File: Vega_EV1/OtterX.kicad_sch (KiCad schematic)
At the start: 62 parts, among them J1 VERA_CONN, J11 KMDGX-6SG, J12 VIA1 Extra Pins, J17 SNES23, J18 SNES0, J19 SNES1, J2 VIA2 Header, J29 AudioPlug3, J3 IEC, J9 I2C, U1 W65C02S, U11 74ACT163, U2 W65C22S, X1 ACH-16.000MHZ-EK

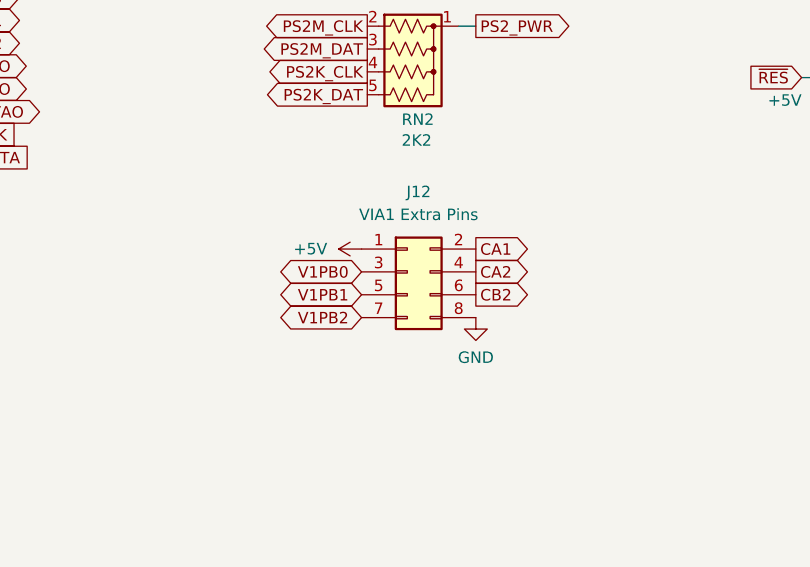
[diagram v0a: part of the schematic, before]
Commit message: Misc layout fixes.
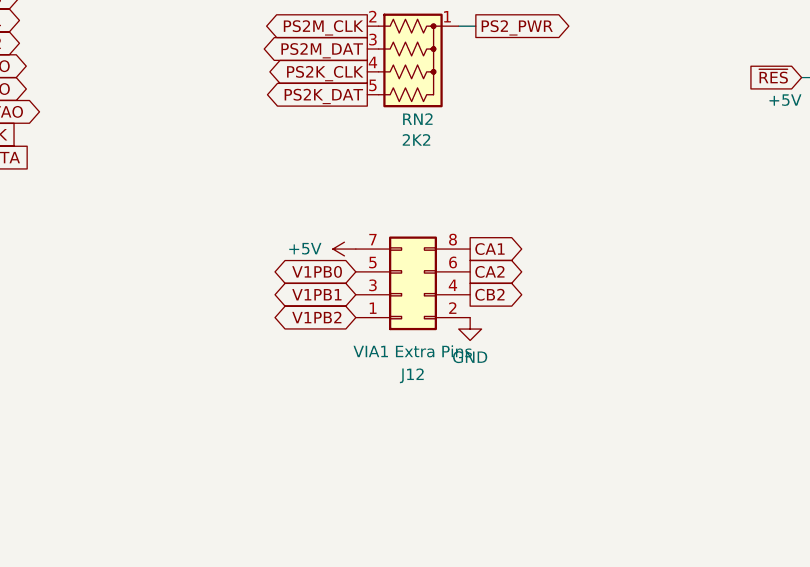
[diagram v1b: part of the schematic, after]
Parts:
- J12: footprint Connector_PinHeader_2.54mm:PinHeader_2x04_P2.54mm_Vertical -> Connector_PinSocket_2.54mm:PinSocket_2x04_P2.54mm_Horizontal
- J17: footprint Connector_PinSocket_2.54mm:PinSocket_2x03_P2.54mm_Vertical -> Connector_PinSocket_2.54mm:PinSocket_2x03_P2.54mm_Horizontal
- J3: footprint Connector_PinHeader_2.54mm:PinHeader_2x05_P2.54mm_Vertical -> Connector_PinSocket_2.54mm:PinSocket_2x05_P2.54mm_Vertical
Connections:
- net +5V: now also J12.7 (Pin_7); no longer J12.1 (Pin_1)
- net CA1: now also J12.8 (Pin_8); no longer J12.2 (Pin_2)
- net CA2: now also J12.6 (Pin_6); no longer J12.4 (Pin_4)
- net CB2: now also J12.4 (Pin_4); no longer J12.6 (Pin_6)
- net GND: now also J12.2 (Pin_2); no longer J12.8 (Pin_8)
- net V1PB0: now also J12.5 (Pin_5); no longer J12.3 (Pin_3)
- net V1PB1: now also J12.3 (Pin_3); no longer J12.5 (Pin_5)
- net V1PB2: now also J12.1 (Pin_1); no longer J12.7 (Pin_7)
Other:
- moved on the sheet: J12
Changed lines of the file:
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@@
 	(global_label "CA1"
 		(shape output)
-		(at 313.055 90.17 0)
+		(at 312.42 90.17 0)
 		(fields_autoplaced yes)
 		(effects
@@
 		)
 		(property "Intersheetrefs" "${INTERSHEET_REFS}"
-			(at 319.5289 90.17 0)
+			(at 318.8939 90.17 0)
 			(effects
 				(font
@@
 	(global_label "CB2"
 		(shape output)
-		(at 313.055 95.25 0)
+		(at 312.42 95.25 0)
 		(fields_autoplaced yes)
 		(effects
@@
 		)
 		(property "Intersheetrefs" "${INTERSHEET_REFS}"
-			(at 319.2176 95.1706 0)
+			(at 318.5826 95.1706 0)
 			(effects
 				(font
@@
 	(global_label "CA2"
 		(shape output)
-		(at 313.055 92.71 0)
+		(at 312.42 92.71 0)
 		(fields_autoplaced yes)
 		(effects
@@
 		)
 		(property "Intersheetrefs" "${INTERSHEET_REFS}"
-			(at 319.5289 92.71 0)
+			(at 318.8939 92.71 0)
 			(effects
 				(font
@@
 	(global_label "V1PB0"
 		(shape bidirectional)
-		(at 300.355 92.71 180)
+		(at 299.72 92.71 180)
 		(fields_autoplaced yes)
 		(effects
@@
 		)
 		(property "Intersheetrefs" "${INTERSHEET_REFS}"
-			(at 291.8943 92.6306 0)
+			(at 291.2593 92.6306 0)
 			(effects
 				(font
@@
 	(global_label "V1PB2"
 		(shape bidirectional)
-		(at 300.355 97.79 180)
+		(at 299.72 97.79 180)
 		(fields_autoplaced yes)
 		(effects
@@
 		)
 		(property "Intersheetrefs" "${INTERSHEET_REFS}"
-			(at 291.8943 97.7106 0)
+			(at 291.2593 97.7106 0)
 			(effects
 				(font
@@
 	(global_label "V1PB1"
 		(shape bidirectional)
-		(at 300.355 95.25 180)
+		(at 299.72 95.25 180)
 		(fields_autoplaced yes)
 		(effects
@@
 		)
 		(property "Intersheetrefs" "${INTERSHEET_REFS}"
-			(at 291.8943 95.1706 0)
+			(at 291.2593 95.1706 0)
 			(effects
 				(font
@@
 	(symbol
 		(lib_id "power:GND")
-		(at 313.055 97.79 0)
+		(at 312.42 97.79 0)
 		(mirror y)
 		(unit 1)
@@
 		(fields_autoplaced yes)
 		(property "Reference" "#PWR010"
-			(at 313.055 104.14 0)
+			(at 312.42 104.14 0)
 			(effects
 				(font
@@
 		)
 		(property "Value" "GND"
-			(at 313.055 102.235 0)
+			(at 312.42 102.235 0)
 			(effects
 				(font
@@
 		)
 		(property "Footprint" ""
-			(at 313.055 97.79 0)
+			(at 312.42 97.79 0)
 			(effects
 				(font
@@
 		)
 		(property "Datasheet" ""
-			(at 313.055 97.79 0)
+			(at 312.42 97.79 0)
 			(effects
 				(font
@@
 		)
 		(property "Description" "Power symbol creates a global label with name \"GND\" , ground"
-			(at 313.055 97.79 0)
+			(at 312.42 97.79 0)
 			(effects
 				(font
@@
 	(symbol
 		(lib_id "power:+5V")
-		(at 300.355 90.17 90)
+		(at 299.72 90.17 90)
 		(mirror x)
 		(unit 1)
@@
 		(fields_autoplaced yes)
 		(property "Reference" "#PWR09"
-			(at 304.165 90.17 0)
+			(at 303.53 90.17 0)
 			(effects
 				(font
@@
 		)
 		(property "Value" "+5V"
-			(at 296.545 90.1699 90)
+			(at 295.91 90.1699 90)
 			(effects
 				(font
@@
 		)
 		(property "Footprint" ""
-			(at 300.355 90.17 0)
+			(at 299.72 90.17 0)
 			(effects
 				(font
@@
 		)
 		(property "Datasheet" ""
-			(at 300.355 90.17 0)
+			(at 299.72 90.17 0)
 			(effects
 				(font
@@
 		)
 		(property "Description" "Power symbol creates a global label with name \"+5V\""
-			(at 300.355 90.17 0)
+			(at 299.72 90.17 0)
 			(effects
 				(font
@@
 		(on_board yes)
 		(dnp no)
-		(fields_autoplaced yes)
 		(property "Reference" "J3"
 			(at 307.34 133.35 0)
@@
 			)
 		)
-		(property "Footprint" "Connector_PinHeader_2.54mm:PinHeader_2x05_P2.54mm_Vertical"
+		(property "Footprint" "Connector_PinSocket_2.54mm:PinSocket_2x05_P2.54mm_Vertical"
 			(at 306.07 144.78 0)
 			(effects
@@
 	(symbol
 		(lib_id "Connector_Generic:Conn_02x04_Odd_Even")
-		(at 305.435 92.71 0)
+		(at 304.8 95.25 0)
+		(mirror x)
 		(unit 1)
 		(exclude_from_sim no)
@@
 		(on_board yes)
 		(dnp no)
-		(fields_autoplaced yes)
 		(property "Reference" "J12"
-			(at 306.705 83.82 0)
+			(at 306.07 104.14 0)
 			(effects
 				(font
@@
 		)
 		(property "Value" "VIA1 Extra Pins"
-			(at 306.705 86.36 0)
+			(at 306.07 101.6 0)
 			(effects
 				(font
@@
 			)
 		)
-		(property "Footprint" "Connector_PinHeader_2.54mm:PinHeader_2x04_P2.54mm_Vertical"
-			(at 305.435 92.71 0)
+		(property "Footprint" "Connector_PinSocket_2.54mm:PinSocket_2x04_P2.54mm_Horizontal"
+			(at 304.8 95.25 0)
 			(effects
 				(font
@@
 		)
 		(property "Datasheet" "~"
-			(at 305.435 92.71 0)
+			(at 304.8 95.25 0)
 			(effects
 				(font
@@
 		)
 		(property "Description" ""
-			(at 305.435 92.71 0)
+			(at 304.8 95.25 0)
 			(effects
 				(font
@@
 			)
 		)
-		(property "Footprint" "Connector_PinSocket_2.54mm:PinSocket_2x03_P2.54mm_Vertical"
+		(property "Footprint" "Connector_PinSocket_2.54mm:PinSocket_2x03_P2.54mm_Horizontal"
 			(at 155.575 229.87 0)
 			(effects
